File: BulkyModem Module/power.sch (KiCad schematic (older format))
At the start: 9 parts, among them J1 DC IN, K1 HK19F-DC, U2 74HCT04

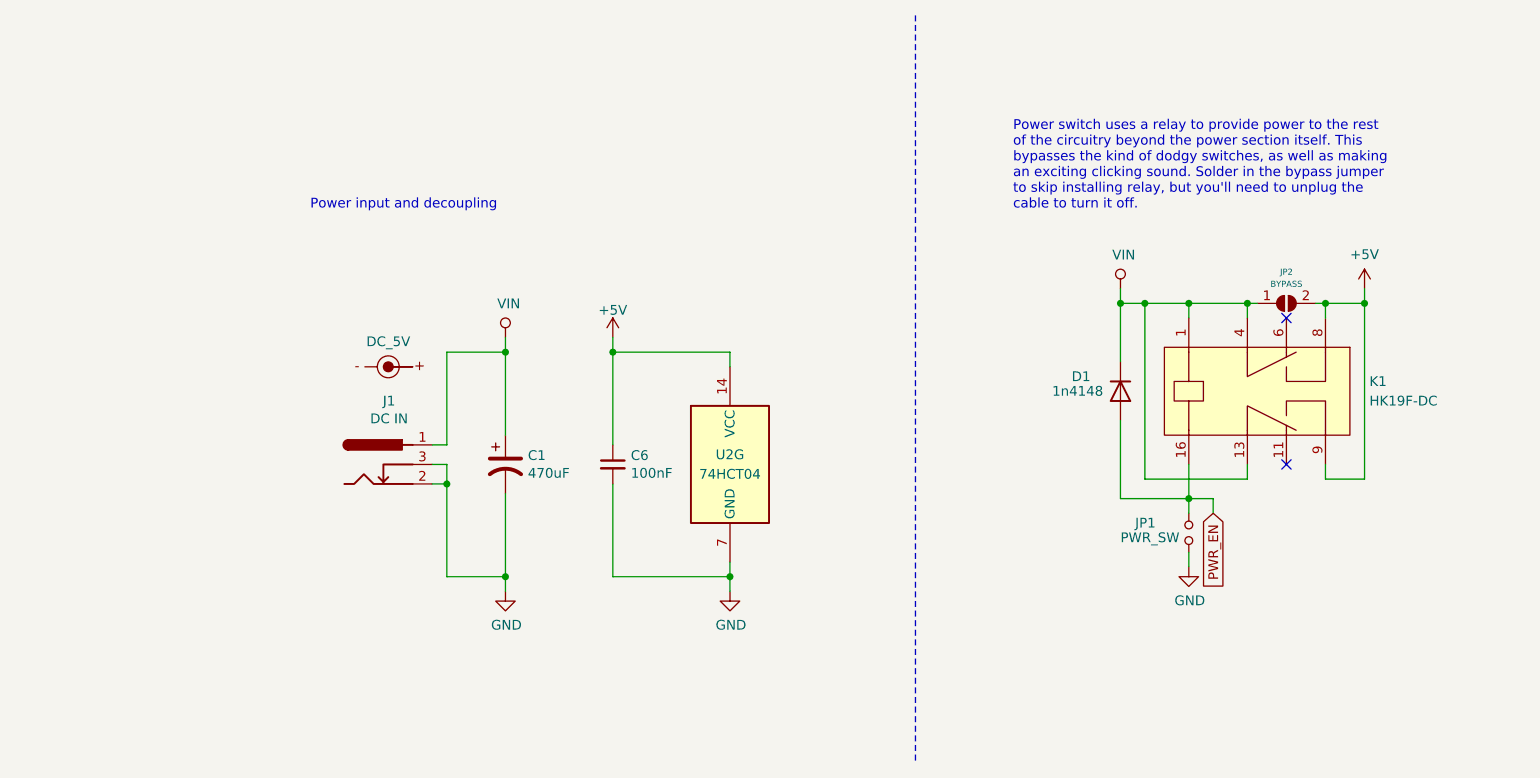
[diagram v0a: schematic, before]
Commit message: Add DCD
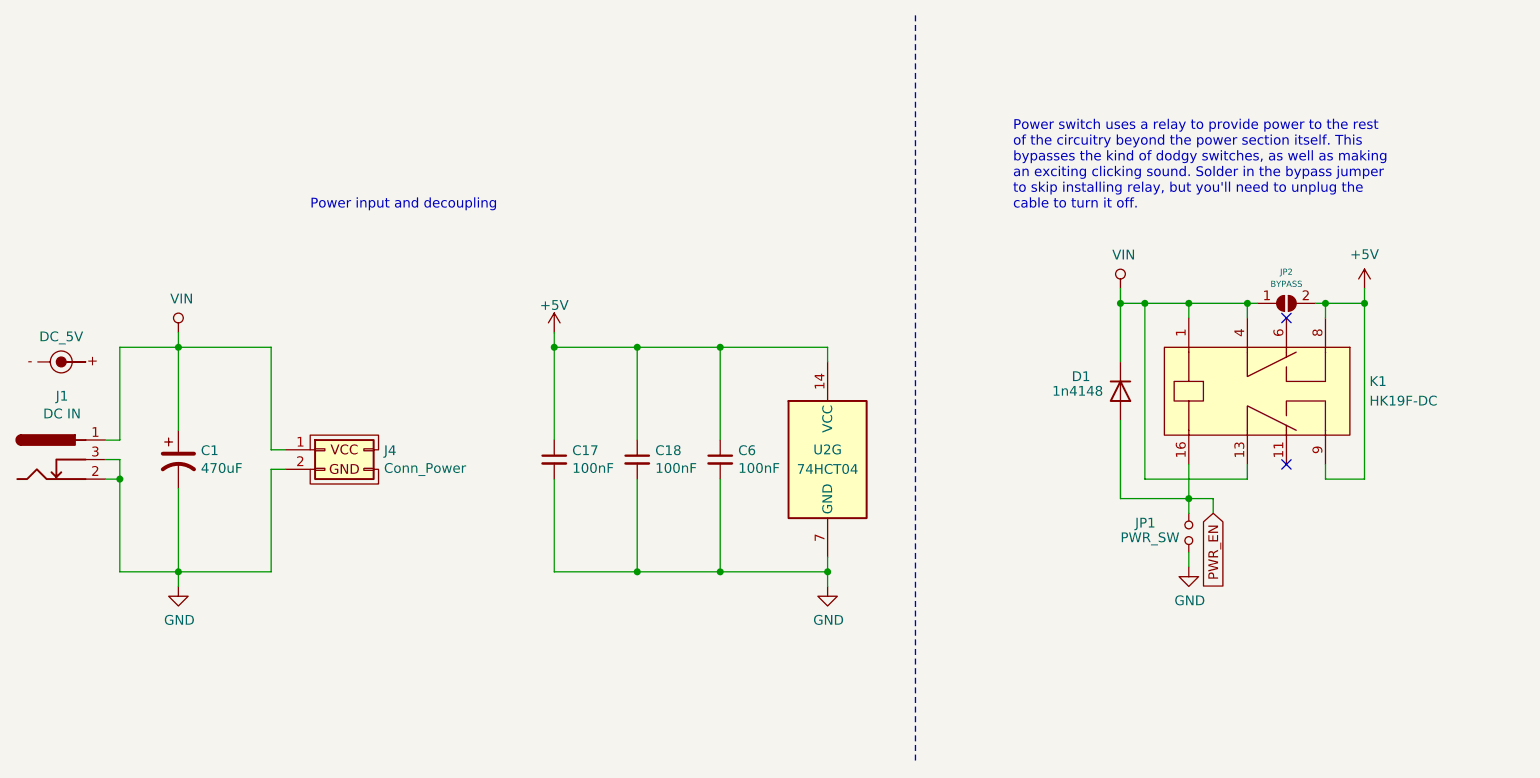
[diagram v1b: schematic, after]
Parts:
- added C17, C18: 100nF, Capacitor_THT:C_Disc_D4.7mm_W2.5mm_P5.00mm, symbol Device:C_Small
- added J4: Conn_Power, BulkyModem:Conn_Power, symbol BulkyModem:Conn_Power
- J1: footprint Connectors:BARREL_JACK -> BulkyModem:BARREL_JACK
- SYM1: footprint BulkyMIDI-32:PWR_Specification -> BulkyModem:PWR_Specification
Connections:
- net +5V: now also C17.1, C18.1
- net GND: now also C17.2, C18.2, J4.2 (GND)
- net VIN: now also J4.1 (VCC)
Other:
- moved on the sheet: C1, C6, J1, U2G
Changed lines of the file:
@@
 L barrel_jack:barrel_9v J?
 U 1 1 63DAB478
-P 3050 4025
+P 1375 4000
 AR Path="/63DAB478" Ref="J?"  Part="1"
 AR Path="/63D786E4/63DAB478" Ref="J1"  Part="1"
-F 0 "J1" H 3129 4350 50  0000 C CNN
-F 1 "DC IN" H 3129 4259 50  0000 C CNN
-F 2 "Connectors:BARREL_JACK" H 3100 3985 50  0001 C CNN
-F 3 "~" H 3100 3985 50  0001 C CNN
-	1    3050 4025
+F 0 "J1" H 1454 4325 50  0000 C CNN
+F 1 "DC IN" H 1454 4234 50  0000 C CNN
+F 2 "BulkyModem:BARREL_JACK" H 1425 3960 50  0001 C CNN
+F 3 "~" H 1425 3960 50  0001 C CNN
+	1    1375 4000
 	1    0    0    -1
 $EndComp
@@
 L power:GND #PWR?
 U 1 1 63DAB47E
-P 3725 4675
+P 2050 4650
 AR Path="/63DAB47E" Ref="#PWR?"  Part="1"
 AR Path="/63D786E4/63DAB47E" Ref="#PWR0108"  Part="1"
-F 0 "#PWR0108" H 3725 4425 50  0001 C CNN
-F 1 "GND" H 3730 4502 50  0000 C CNN
-F 2 "" H 3725 4675 50  0001 C CNN
-F 3 "" H 3725 4675 50  0001 C CNN
-	1    3725 4675
+F 0 "#PWR0108" H 2050 4400 50  0001 C CNN
+F 1 "GND" H 2055 4477 50  0000 C CNN
+F 2 "" H 2050 4650 50  0001 C CNN
+F 3 "" H 2050 4650 50  0001 C CNN
+	1    2050 4650
 	1    0    0    -1
 $EndComp
@@
 L Device:C_Small C?
 U 1 1 63DAB484
-P 4275 4025
+P 4825 4000
 AR Path="/63DAB484" Ref="C?"  Part="1"
 AR Path="/63D786E4/63DAB484" Ref="C6"  Part="1"
-F 0 "C6" H 4367 4071 50  0000 L CNN
-F 1 "100nF" H 4367 3980 50  0000 L CNN
-F 2 "Capacitor_THT:C_Disc_D4.7mm_W2.5mm_P5.00mm" H 4275 4025 50  0001 C CNN
-F 3 "~" H 4275 4025 50  0001 C CNN
-	1    4275 4025
-	1    0    0    -1
-$EndComp
-Wire Wire Line
-	3350 3925 3425 3925
-Wire Wire Line
-	3350 4125 3425 4125
+F 0 "C6" H 4917 4046 50  0000 L CNN
+F 1 "100nF" H 4917 3955 50  0000 L CNN
+F 2 "Capacitor_THT:C_Disc_D4.7mm_W2.5mm_P5.00mm" H 4825 4000 50  0001 C CNN
+F 3 "~" H 4825 4000 50  0001 C CNN
+	1    4825 4000
+	1    0    0    -1
+$EndComp
+Wire Wire Line
+	1675 3900 1750 3900
+Wire Wire Line
+	1675 4100 1750 4100
 $Comp
 L Device:CP1 C?
 U 1 1 63DAB48C
-P 3725 4025
+P 2050 4000
 AR Path="/63DAB48C" Ref="C?"  Part="1"
 AR Path="/63D786E4/63DAB48C" Ref="C1"  Part="1"
-F 0 "C1" H 3840 4071 50  0000 L CNN
-F 1 "470uF" H 3840 3980 50  0000 L CNN
-F 2 "Capacitor_THT:CP_Radial_D8.0mm_P3.50mm" H 3725 4025 50  0001 C CNN
-F 3 "~" H 3725 4025 50  0001 C CNN
-	1    3725 4025
+F 0 "C1" H 2165 4046 50  0000 L CNN
+F 1 "470uF" H 2165 3955 50  0000 L CNN
+F 2 "Capacitor_THT:CP_Radial_D8.0mm_P3.50mm" H 2050 4000 50  0001 C CNN
+F 3 "~" H 2050 4000 50  0001 C CNN
+	1    2050 4000
 	1    0    0    -1
 $EndComp
@@
 L power:+5V #PWR?
 U 1 1 63DAB492
-P 4275 3375
+P 3975 3350
 AR Path="/63DAB492" Ref="#PWR?"  Part="1"
 AR Path="/63D786E4/63DAB492" Ref="#PWR0110"  Part="1"
-F 0 "#PWR0110" H 4275 3225 50  0001 C CNN
-F 1 "+5V" H 4275 3515 50  0000 C CNN
-F 2 "" H 4275 3375 50  0000 C CNN
-F 3 "" H 4275 3375 50  0000 C CNN
-	1    4275 3375
-	1    0    0    -1
-$EndComp
-Wire Wire Line
-	4875 4600 4875 4525
+F 0 "#PWR0110" H 3975 3200 50  0001 C CNN
+F 1 "+5V" H 3975 3490 50  0000 C CNN
+F 2 "" H 3975 3350 50  0000 C CNN
+F 3 "" H 3975 3350 50  0000 C CNN
+	1    3975 3350
+	1    0    0    -1
+$EndComp
+Wire Wire Line
+	5375 4575 5375 4500
 $Comp
 L power:GND #PWR?
 U 1 1 63DAB499
-P 4875 4675
+P 5375 4650
 AR Path="/63DAB499" Ref="#PWR?"  Part="1"
 AR Path="/63D786E4/63DAB499" Ref="#PWR0133"  Part="1"
-F 0 "#PWR0133" H 4875 4425 50  0001 C CNN
-F 1 "GND" H 4880 4502 50  0000 C CNN
-F 2 "" H 4875 4675 50  0001 C CNN
-F 3 "" H 4875 4675 50  0001 C CNN
-	1    4875 4675
-	1    0    0    -1
-$EndComp
-Wire Wire Line
-	4275 4125 4275 4600
-Wire Wire Line
-	4275 3450 4275 3925
-Wire Wire Line
-	4875 3450 4875 3525
-Wire Wire Line
-	4275 3375 4275 3450
-Connection ~ 4275 3450
-Wire Wire Line
-	3350 4025 3425 4025
-Wire Wire Line
-	3425 4025 3425 4125
-Connection ~ 3425 4125
-Wire Wire Line
-	3725 3375 3725 3450
-Wire Wire Line
-	3725 3450 3425 3450
-Connection ~ 3725 3450
-Wire Wire Line
-	3425 3450 3425 3925
-Wire Wire Line
-	3725 3450 3725 3875
-Wire Wire Line
-	3725 4600 3425 4600
-Connection ~ 3725 4600
-Wire Wire Line
-	3725 4600 3725 4675
-Wire Wire Line
-	3425 4125 3425 4600
-Wire Wire Line
-	3725 4175 3725 4600
+F 0 "#PWR0133" H 5375 4400 50  0001 C CNN
+F 1 "GND" H 5380 4477 50  0000 C CNN
+F 2 "" H 5375 4650 50  0001 C CNN
+F 3 "" H 5375 4650 50  0001 C CNN
+	1    5375 4650
+	1    0    0    -1
+$EndComp
+Wire Wire Line
+	4825 4100 4825 4575
+Wire Wire Line
+	4825 3425 4825 3900
+Wire Wire Line
+	5375 3425 5375 3500
+Wire Wire Line
+	3975 3350 3975 3425
+Wire Wire Line
+	1675 4000 1750 4000
+Wire Wire Line
+	1750 4000 1750 4100
+Connection ~ 1750 4100
+Wire Wire Line
+	2050 3350 2050 3425
+Wire Wire Line
+	2050 3425 1750 3425
+Connection ~ 2050 3425
+Wire Wire Line
+	1750 3425 1750 3900
+Wire Wire Line
+	2050 3425 2050 3850
+Wire Wire Line
+	2050 4575 1750 4575
+Connection ~ 2050 4575
+Wire Wire Line
+	2050 4575 2050 4650
+Wire Wire Line
+	1750 4100 1750 4575
+Wire Wire Line
+	2050 4150 2050 4575
 $Comp
 L BulkyModem:DC_5V SYM?
 U 1 1 63DAB4B1
-P 3125 3525
+P 1450 3500
 AR Path="/63DAB4B1" Ref="SYM?"  Part="1"
 AR Path="/63D786E4/63DAB4B1" Ref="SYM1"  Part="1"
-F 0 "SYM1" H 3125 3746 50  0001 C CNN
-F 1 "DC_5V" H 3125 3654 50  0000 C CNN
-F 2 "BulkyMIDI-32:PWR_Specification" H 3000 3625 50  0001 C CNN
-F 3 "" H 3000 3625 50  0001 C CNN
-	1    3125 3525
+F 0 "SYM1" H 1450 3721 50  0001 C CNN
+F 1 "DC_5V" H 1450 3629 50  0000 C CNN
+F 2 "BulkyModem:PWR_Specification" H 1325 3600 50  0001 C CNN
+F 3 "" H 1325 3600 50  0001 C CNN
+	1    1450 3500
 	1    0    0    -1
 $EndComp
 Text Notes 2725 2725 0    50   ~ 0
 Power input and decoupling
-Wire Wire Line
-	4275 4600 4875 4600
 $Comp
 L barrel_jack:VIN #PWR?
 U 1 1 63DAB4BE
-P 3725 3375
+P 2050 3350
 AR Path="/63DAB4BE" Ref="#PWR?"  Part="1"
 AR Path="/63D786E4/63DAB4BE" Ref="#PWR0134"  Part="1"
-F 0 "#PWR0134" H 3725 3225 50  0001 C CNN
-F 1 "VIN" H 3742 3548 50  0000 C CNN
-F 2 "" H 3725 3375 50  0001 C CNN
-F 3 "" H 3725 3375 50  0001 C CNN
-	1    3725 3375
+F 0 "#PWR0134" H 2050 3200 50  0001 C CNN
+F 1 "VIN" H 2067 3523 50  0000 C CNN
+F 2 "" H 2050 3350 50  0001 C CNN
+F 3 "" H 2050 3350 50  0001 C CNN
+	1    2050 3350
 	1    0    0    -1
 $EndComp
@@
 L 74xx:74HCT04 U?
 U 7 1 63DAB4C4
-P 4875 4025
+P 5375 4000
 AR Path="/63DAB4C4" Ref="U?"  Part="7"
 AR Path="/63D786E4/63DAB4C4" Ref="U2"  Part="7"
-F 0 "U2" H 4875 4075 50  0000 C CNN
-F 1 "74HCT04" H 4875 3975 50  0000 C CNN
-F 2 "Package_DIP:DIP-14_W7.62mm_Socket_LongPads" H 4875 4025 50  0001 C CNN
-F 3 "https://assets.nexperia.com/documents/data-sheet/74HC_HCT04.pdf" H 4875 4025 50  0001 C CNN
-	7    4875 4025
-	1    0    0    -1
-$EndComp
-Wire Wire Line
-	4875 3450 4275 3450
-Wire Wire Line
-	4875 4675 4875 4600
-Connection ~ 4875 4600
+F 0 "U2" H 5375 4050 50  0000 C CNN
+F 1 "74HCT04" H 5375 3950 50  0000 C CNN
+F 2 "Package_DIP:DIP-14_W7.62mm_Socket_LongPads" H 5375 4000 50  0001 C CNN
+F 3 "https://assets.nexperia.com/documents/data-sheet/74HC_HCT04.pdf" H 5375 4000 50  0001 C CNN
+	7    5375 4000
+	1    0    0    -1
+$EndComp
+Wire Wire Line
+	5375 3425 4825 3425
+Wire Wire Line
+	5375 4650 5375 4575
+Connection ~ 5375 4575
 Text Notes 6325 2725 0    50   ~ 0
 Power switch uses a relay to provide power to the rest\nof the circuitry beyond the power section itself. This\nbypasses the kind of dodgy switches, as well as making\nan exciting clicking sound. Solder in the bypass jumper\nto skip installing relay, but you'll need to unplug the\ncable to turn it off.
 Wire Notes Line
 	5825 1725 5825 5550
+$Comp
+L BulkyModem:Conn_Power J4
+U 1 1 62DFBB40
+P 2800 3950
+F 0 "J4" H 3103 3946 50  0000 L CNN
+F 1 "Conn_Power" H 3103 3855 50  0000 L CNN
+F 2 "BulkyModem:Conn_Power" H 2800 3950 50  0001 C CNN
+F 3 "~" H 2800 3950 50  0001 C CNN
+	1    2800 3950
+	1    0    0    -1
+$EndComp
+Wire Wire Line
+	2050 3425 2525 3425
+Wire Wire Line
+	2525 3425 2525 3950
+Wire Wire Line
+	2525 3950 2600 3950
+Wire Wire Line
+	2600 4050 2525 4050
+Wire Wire Line
+	2525 4050 2525 4575
+Wire Wire Line
+	2525 4575 2050 4575
+$Comp
+L Device:C_Small C?
+U 1 1 6319B9B5
+P 4400 4000
+AR Path="/6319B9B5" Ref="C?"  Part="1"
+AR Path="/63D786E4/6319B9B5" Ref="C18"  Part="1"
+F 0 "C18" H 4492 4046 50  0000 L CNN
+F 1 "100nF" H 4492 3955 50  0000 L CNN
+F 2 "Capacitor_THT:C_Disc_D4.7mm_W2.5mm_P5.00mm" H 4400 4000 50  0001 C CNN
+F 3 "~" H 4400 4000 50  0001 C CNN
+	1    4400 4000
+	1    0    0    -1
+$EndComp
+Wire Wire Line
+	4400 4100 4400 4575
+Wire Wire Line
+	4400 3425 4400 3900
+$Comp
+L Device:C_Small C?
+U 1 1 6319CE6C
+P 3975 4000
+AR Path="/6319CE6C" Ref="C?"  Part="1"
+AR Path="/63D786E4/6319CE6C" Ref="C17"  Part="1"
+F 0 "C17" H 4067 4046 50  0000 L CNN
+F 1 "100nF" H 4067 3955 50  0000 L CNN
+F 2 "Capacitor_THT:C_Disc_D4.7mm_W2.5mm_P5.00mm" H 3975 4000 50  0001 C CNN
+F 3 "~" H 3975 4000 50  0001 C CNN
+	1    3975 4000
+	1    0    0    -1
+$EndComp
+Wire Wire Line
+	3975 4100 3975 4575
+Wire Wire Line
+	3975 3425 3975 3900
+Connection ~ 4825 3425
+Connection ~ 4825 4575
+Wire Wire Line
+	4825 4575 5375 4575
+Connection ~ 4400 3425
+Wire Wire Line
+	4400 3425 3975 3425
+Wire Wire Line
+	3975 4575 4400 4575
+Connection ~ 4400 4575
+Wire Wire Line
+	4400 4575 4825 4575
+Connection ~ 3975 3425
+Wire Wire Line
+	4400 3425 4825 3425
 $EndSCHEMATC
